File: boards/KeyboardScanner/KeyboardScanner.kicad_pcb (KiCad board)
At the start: 2 copper layers, 150 x 100 mm, 36 parts, among them J1 Keyboard1, J2 Keyboard1, J3 Encoder, J4 Select, U1 74LS151, U10 74LS151, U2 74LS151, U3 74LS151, U4 74LS151, U5 ULN2803A, U6 74LS151, U7 74LS151, U8 4069, U9 74LS151

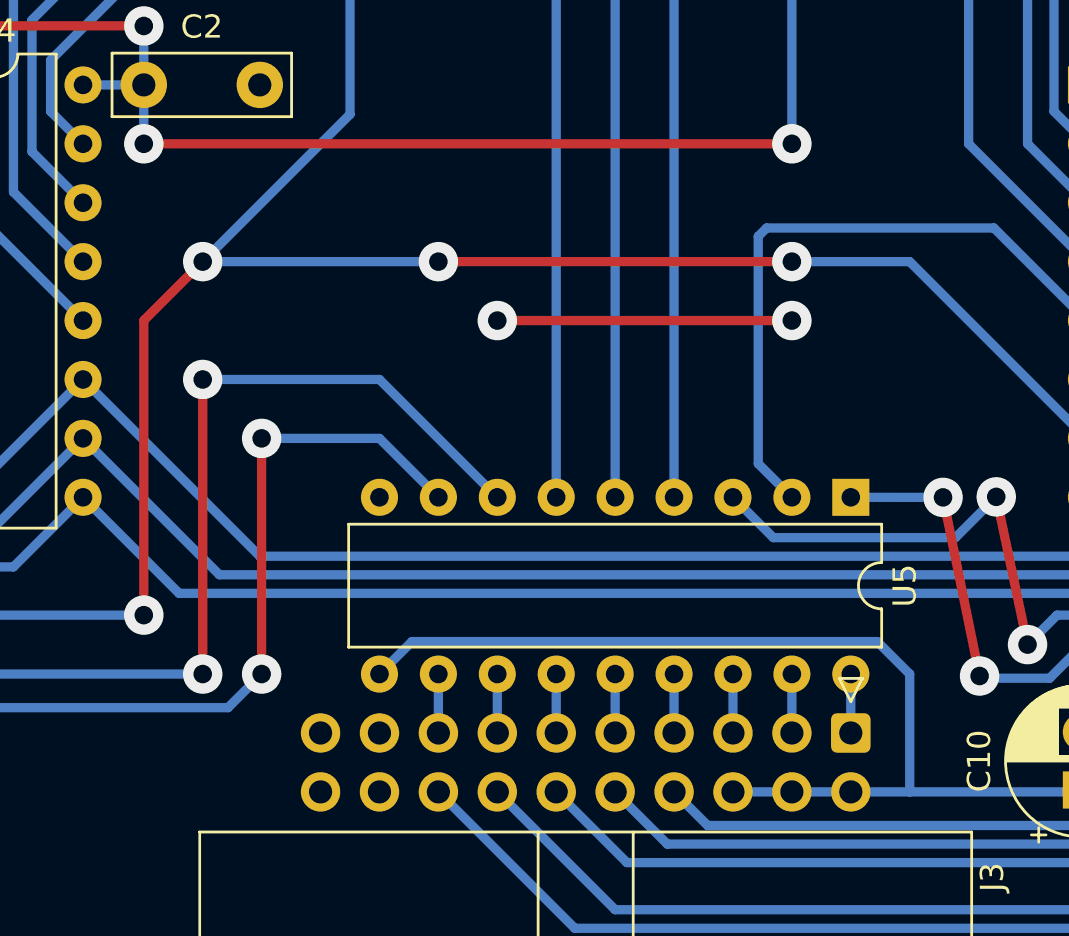
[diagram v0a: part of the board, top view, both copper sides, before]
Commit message: Replaced inverting with non-inverting output buffer in KeyboardScanner to fix disabled open collector output
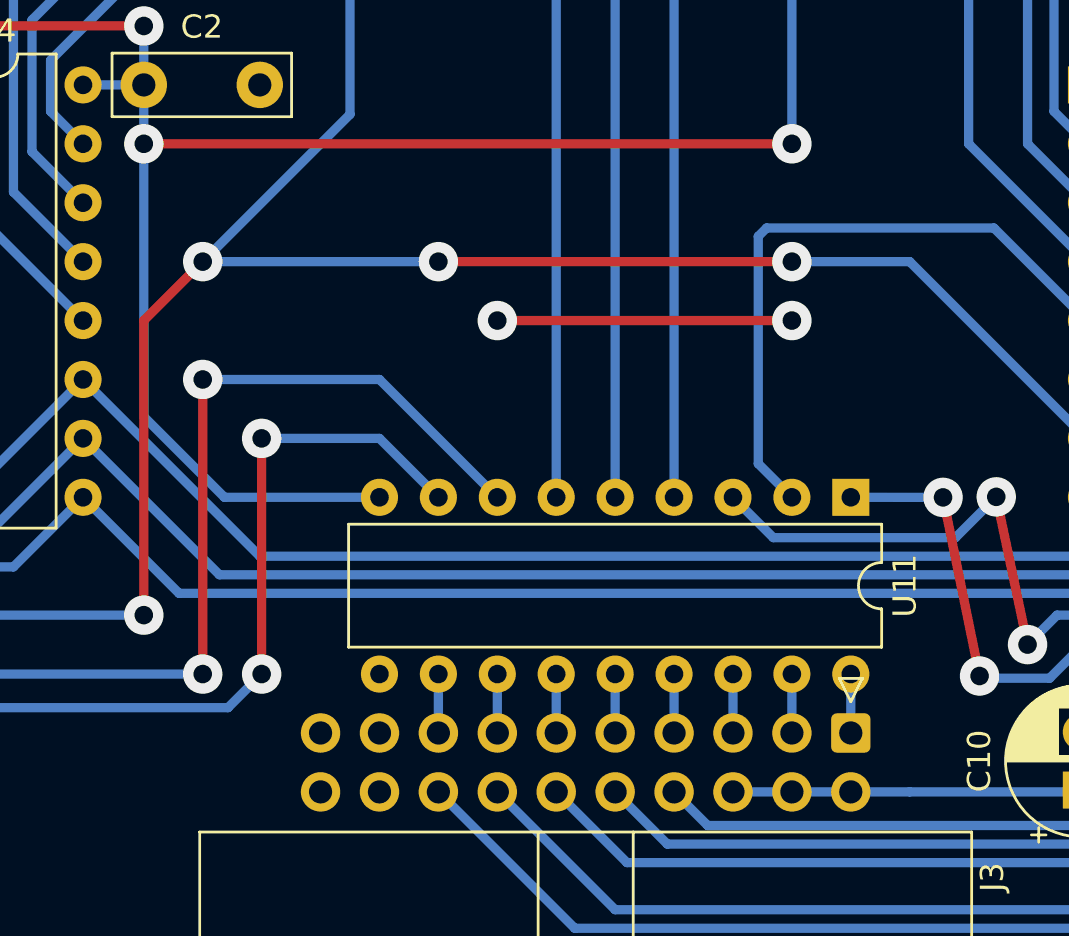
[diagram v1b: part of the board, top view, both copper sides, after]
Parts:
- removed U5: ULN2803A, Package_DIP:DIP-18_W7.62mm
- added U11: TBD62783A, Package_DIP:DIP-18_W7.62mm, F.Cu at (162.6, 119.4)
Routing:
- net +5V: track 368.2 -> 362.4 mm

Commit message: Revert "Replaced inverting with non-inverting output buffer in KeyboardScanner to fix disabled open collector output"
This reverts commit 6ddf25a0a7a31b9f16f3f110cd3b7ae66d122c97.
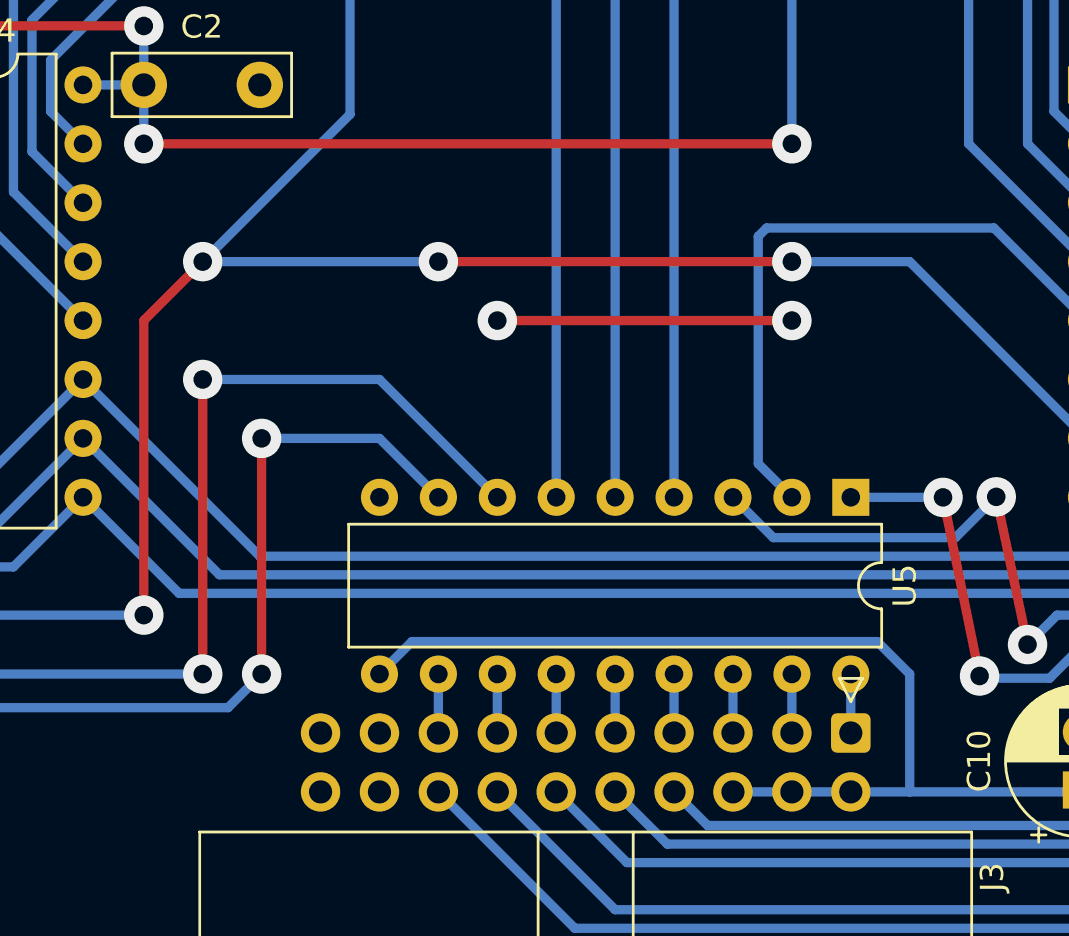
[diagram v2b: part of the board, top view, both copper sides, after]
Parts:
- removed U11: TBD62783A, Package_DIP:DIP-18_W7.62mm
- added U5: ULN2803A, Package_DIP:DIP-18_W7.62mm, F.Cu at (162.6, 119.4)
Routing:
- net +5V: track 362.4 -> 368.2 mm
